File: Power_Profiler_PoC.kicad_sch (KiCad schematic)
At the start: 0 parts

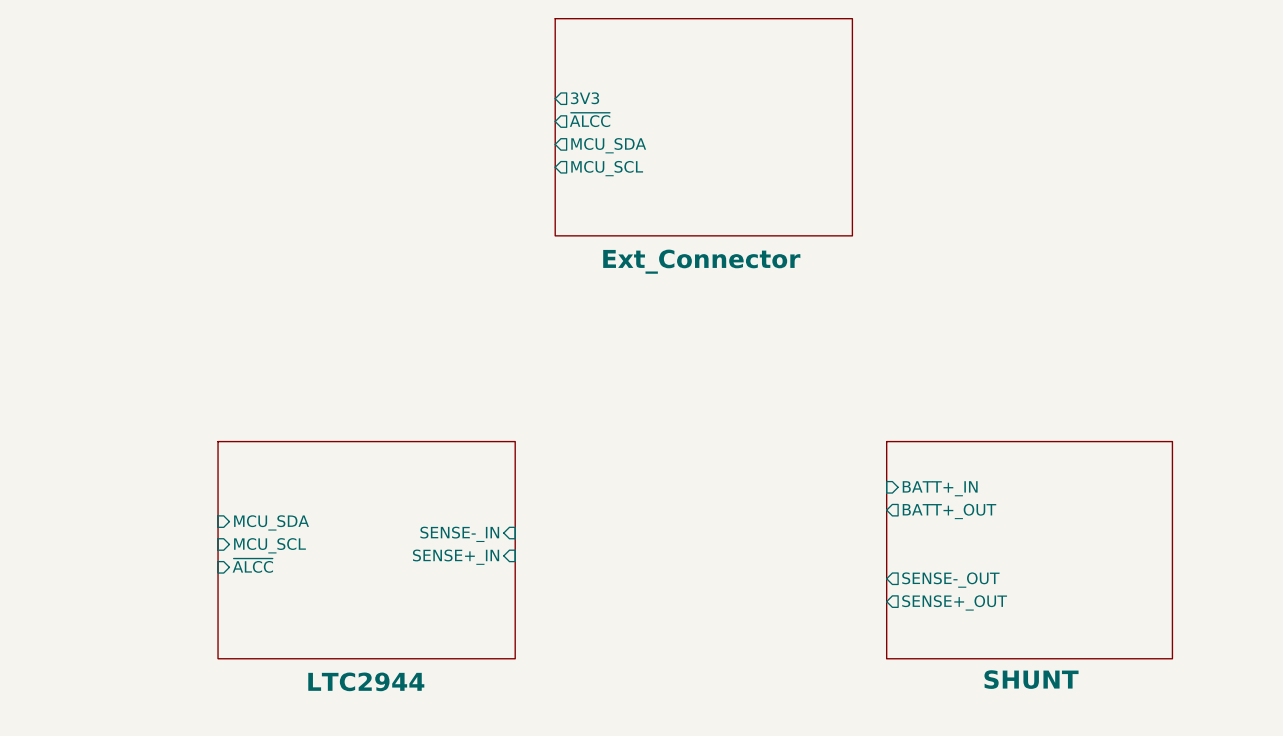
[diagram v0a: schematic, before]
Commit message: Started routing
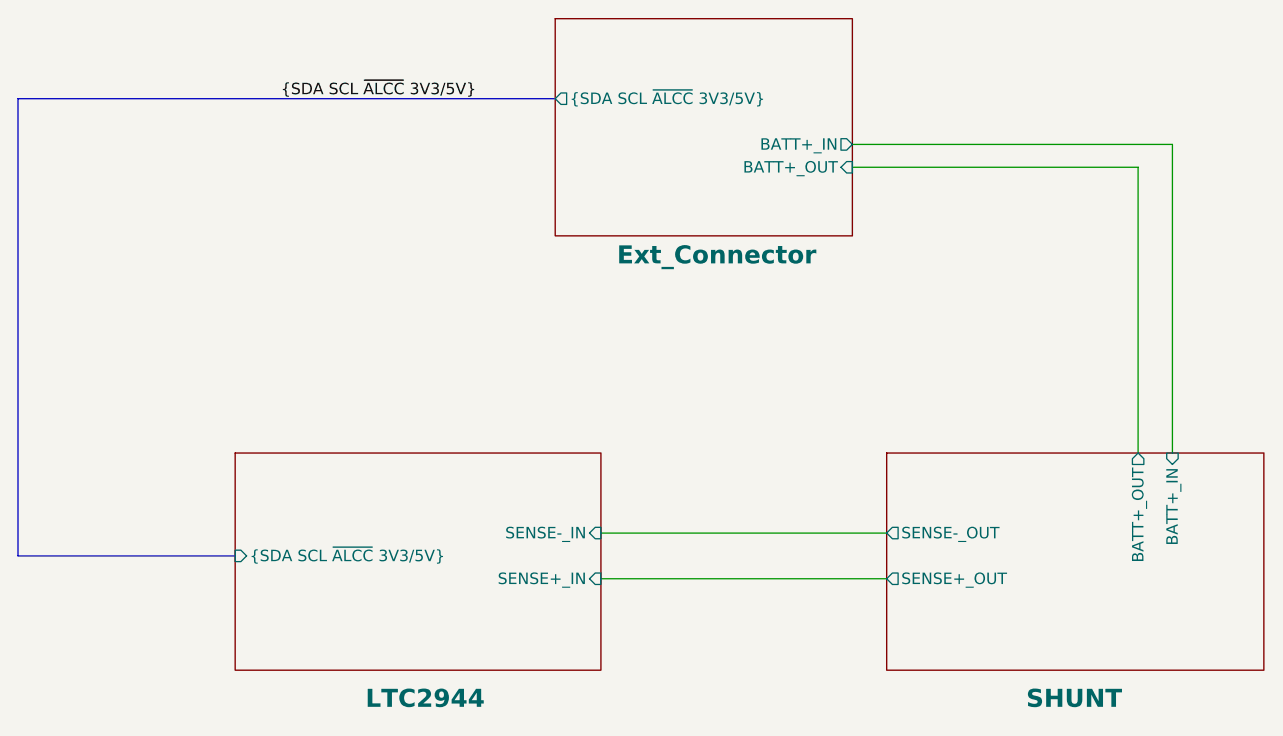
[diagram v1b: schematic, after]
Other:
- sheet Ext_Connector ports: added BATT+_IN, BATT+_OUT, {SDA SCL ~{ALCC} 3V3/5V}; removed 3V3, MCU_SCL, MCU_SDA, ~{ALCC}
- sheet LTC2944 ports: added {SDA SCL ~{ALCC} 3V3/5V}; removed MCU_SCL, MCU_SDA, ~{ALCC}
- sheet SHUNT: file Shunt.kicad_sch -> SHUNT.kicad_sch
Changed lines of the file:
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@@
 		(comment 4 "Author: Vaibhav Khatri")
 	)
+	(bus
+		(pts
+			(xy 137.16 57.15) (xy 77.47 57.15)
+		)
+		(stroke
+			(width 0)
+			(type default)
+		)
+	)
+	(wire
+		(pts
+			(xy 205.74 96.52) (xy 205.74 62.23)
+		)
+		(stroke
+			(width 0.6)
+			(type default)
+		)
+	)
+	(bus
+		(pts
+			(xy 77.47 107.95) (xy 101.6 107.95)
+		)
+		(stroke
+			(width 0)
+			(type default)
+		)
+	)
+	(wire
+		(pts
+			(xy 201.93 64.77) (xy 201.93 96.52)
+		)
+		(stroke
+			(width 0.6)
+			(type default)
+		)
+	)
+	(wire
+		(pts
+			(xy 170.18 64.77) (xy 201.93 64.77)
+		)
+		(stroke
+			(width 0.6)
+			(type default)
+		)
+	)
+	(bus
+		(pts
+			(xy 77.47 57.15) (xy 77.47 107.95)
+		)
+		(stroke
+			(width 0)
+			(type default)
+		)
+	)
+	(wire
+		(pts
+			(xy 205.74 62.23) (xy 170.18 62.23)
+		)
+		(stroke
+			(width 0.6)
+			(type default)
+		)
+	)
+	(wire
+		(pts
+			(xy 142.24 110.49) (xy 173.99 110.49)
+		)
+		(stroke
+			(width 0.6)
+			(type default)
+		)
+	)
+	(wire
+		(pts
+			(xy 142.24 105.41) (xy 173.99 105.41)
+		)
+		(stroke
+			(width 0.6)
+			(type default)
+		)
+	)
+	(label "{SDA SCL ~{ALCC} 3V3{slash}5V}"
+		(at 106.68 57.15 0)
+		(fields_autoplaced yes)
+		(effects
+			(font
+				(size 1.27 1.27)
+			)
+			(justify left bottom)
+		)
+	)
 	(sheet
-		(at 99.695 95.25)
-		(size 33.02 24.13)
+		(at 101.6 96.52)
+		(size 40.64 24.13)
 		(stroke
 			(width 0.1524)
@@
 		)
 		(property "Sheetname" "LTC2944"
-			(at 109.474 123.19 0)
+			(at 116.078 124.968 0)
 			(effects
 				(font
 					(size 2 2)
 					(bold yes)
-					(color 0 0 255 1)
+					(color 0 0 0 1)
 				)
 				(justify left bottom)
@@
 		)
 		(property "Sheetfile" "LTC2944.kicad_sch"
-			(at 99.695 119.9646 0)
+			(at 101.6 121.2346 0)
 			(effects
 				(font
@@
 		)
 		(pin "SENSE-_IN" input
-			(at 132.715 105.41 0)
+			(at 142.24 105.41 0)
 			(effects
 				(font
@@
 		)
 		(pin "SENSE+_IN" input
-			(at 132.715 107.95 0)
-			(effects
-				(font
-					(size 1.27 1.27)
-				)
-				(justify right)
-			)
-		)
-		(pin "MCU_SDA" input
-			(at 99.695 104.14 180)
-			(effects
-				(font
-					(size 1.27 1.27)
-				)
-				(justify left)
-			)
-		)
-		(pin "MCU_SCL" input
-			(at 99.695 106.68 180)
-			(effects
-				(font
-					(size 1.27 1.27)
-				)
-				(justify left)
-			)
-		)
-		(pin "~{ALCC}" input
-			(at 99.695 109.22 180)
+			(at 142.24 110.49 0)
+			(effects
+				(font
+					(size 1.27 1.27)
+				)
+				(justify right)
+			)
+		)
+		(pin "{SDA SCL ~{ALCC} 3V3{slash}5V}" input
+			(at 101.6 107.95 180)
 			(effects
 				(font
@@
 	)
 	(sheet
-		(at 173.99 95.25)
-		(size 31.75 24.13)
+		(at 173.99 96.52)
+		(size 41.91 24.13)
 		(stroke
 			(width 0.1524)
@@
 		)
 		(property "Sheetname" "SHUNT"
-			(at 184.658 122.936 0)
+			(at 189.484 124.968 0)
 			(effects
 				(font
 					(size 2 2)
 					(bold yes)
-					(color 0 0 255 1)
+					(color 0 0 0 1)
 				)
 				(justify left bottom)
 			)
 		)
-		(property "Sheetfile" "Shunt.kicad_sch"
-			(at 173.99 119.9646 0)
+		(property "Sheetfile" "SHUNT.kicad_sch"
+			(at 173.99 121.2346 0)
 			(effects
 				(font
@@
 			)
 		)
+		(pin "SENSE+_OUT" output
+			(at 173.99 110.49 180)
+			(effects
+				(font
+					(size 1.27 1.27)
+				)
+				(justify left)
+			)
+		)
+		(pin "BATT+_OUT" output
+			(at 201.93 96.52 90)
+			(effects
+				(font
+					(size 1.27 1.27)
+				)
+				(justify right)
+			)
+		)
+		(pin "SENSE-_OUT" output
+			(at 173.99 105.41 180)
+			(effects
+				(font
+					(size 1.27 1.27)
+				)
+				(justify left)
+			)
+		)
 		(pin "BATT+_IN" input
-			(at 173.99 100.33 180)
-			(effects
-				(font
-					(size 1.27 1.27)
-				)
-				(justify left)
-			)
-		)
-		(pin "SENSE-_OUT" output
-			(at 173.99 110.49 180)
-			(effects
-				(font
-					(size 1.27 1.27)
-				)
-				(justify left)
-			)
-		)
-		(pin "SENSE+_OUT" output
-			(at 173.99 113.03 180)
-			(effects
-				(font
-					(size 1.27 1.27)
-				)
-				(justify left)
-			)
-		)
-		(pin "BATT+_OUT" output
-			(at 173.99 102.87 180)
-			(effects
-				(font
-					(size 1.27 1.27)
-				)
-				(justify left)
+			(at 205.74 96.52 90)
+			(effects
+				(font
+					(size 1.27 1.27)
+				)
+				(justify right)
 			)
 		)
@@
 			(project "Power_Profiler_PoC"
 				(path "/faeaf365-a06a-4014-84f4-b3c47881c674"
-					(page "3")
+					(page "4")
 				)
 			)
@@
 		)
 		(property "Sheetname" "Ext_Connector"
-			(at 142.24 76.2 0)
+			(at 144.018 75.692 0)
 			(effects
 				(font
 					(size 2 2)
 					(bold yes)
-					(color 0 0 255 1)
+					(color 0 0 0 1)
 				)
 				(justify left bottom)
@@
 			)
 		)
-		(pin "3V3" output
+		(pin "BATT+_OUT" input
+			(at 170.18 64.77 0)
+			(effects
+				(font
+					(size 1.27 1.27)
+				)
+				(justify right)
+			)
+		)
+		(pin "BATT+_IN" output
+			(at 170.18 62.23 0)
+			(effects
+				(font
+					(size 1.27 1.27)
+				)
+				(justify right)
+			)
+		)
+		(pin "{SDA SCL ~{ALCC} 3V3{slash}5V}" output
 			(at 137.16 57.15 180)
 			(effects
 				(font
-					(size 1.27 1.27)
-				)
-				(justify left)
-			)
-		)
-		(pin "~{ALCC}" output
-			(at 137.16 59.69 180)
-			(effects
-				(font
-					(size 1.27 1.27)
-				)
-				(justify left)
-			)
-		)
-		(pin "MCU_SDA" output
-			(at 137.16 62.23 180)
-			(effects
-				(font
-					(size 1.27 1.27)
-				)
-				(justify left)
-			)
-		)
-		(pin "MCU_SCL" output
-			(at 137.16 64.77 180)
-			(effects
-				(font
